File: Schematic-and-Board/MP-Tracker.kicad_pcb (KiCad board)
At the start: 2 copper layers, 61 parts, among them P1 DIL10, Q1 BC817, Q2 IRFR5303, Q3 BC817-40, Q4 IRFR5303, U1 MC34063, U2 TL082, U3 ATMEGA8-AI, U4 MC78L033, X1 3.6864MHz

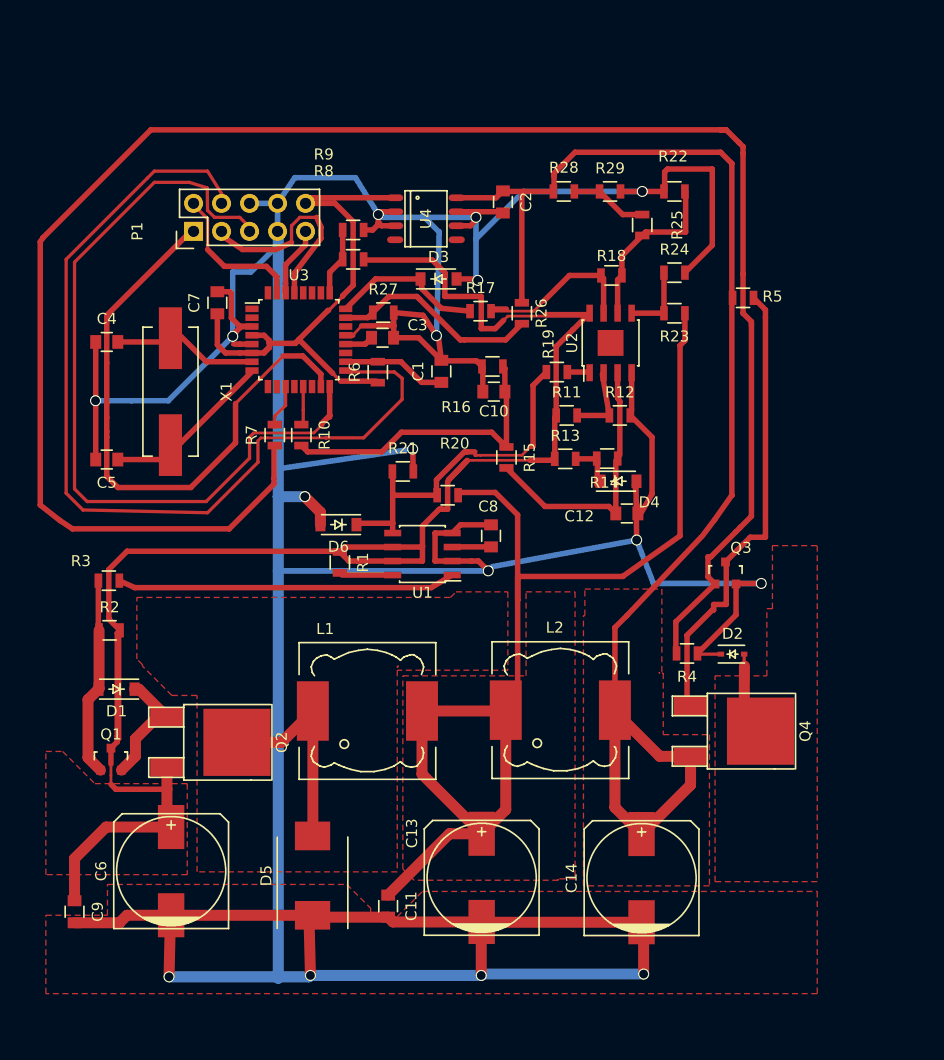
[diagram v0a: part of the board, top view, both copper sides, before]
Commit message: Update schematic and board design and firmware source.
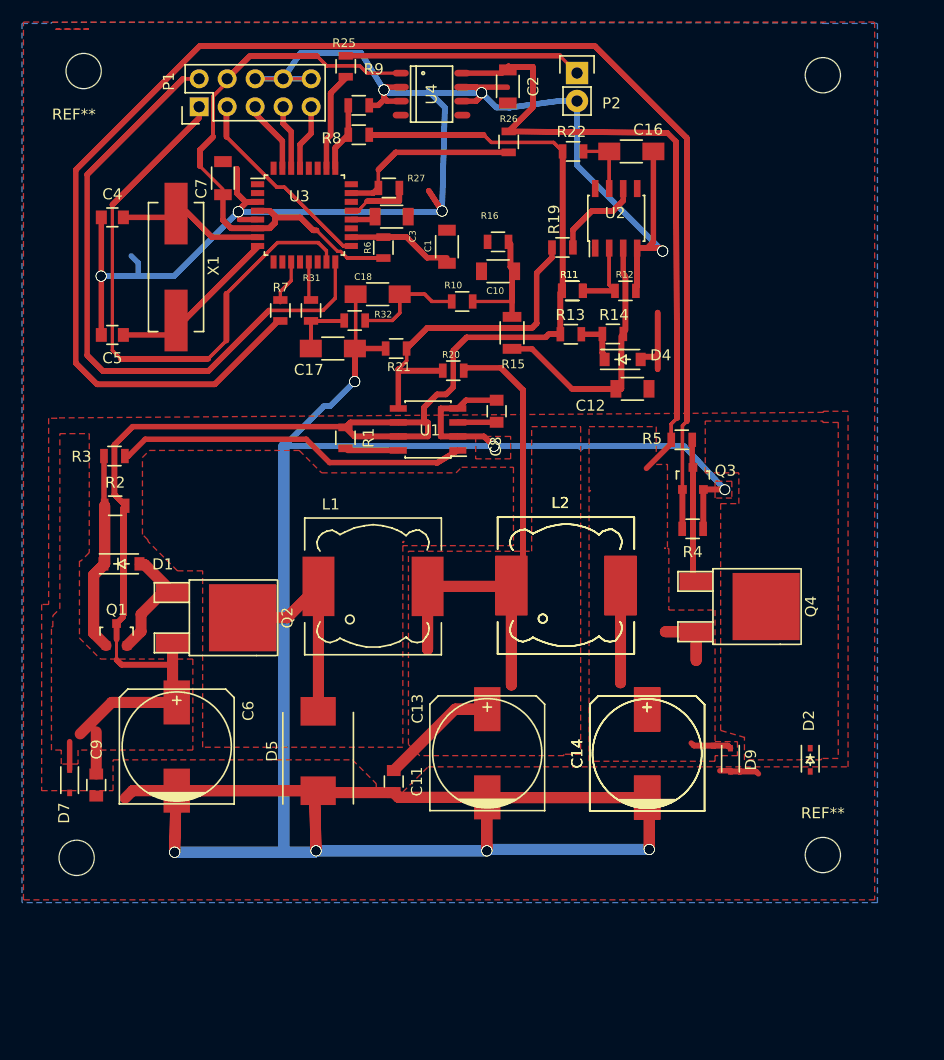
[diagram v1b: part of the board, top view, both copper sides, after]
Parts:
- removed D3, D6: 3V3, Diodes_SMD:SOD-123
- removed R17: 1k, Resistors_SMD:R_0805
- removed R18, R23, R24, R28, R29: 22k, Resistors_SMD:R_0805
- added ?: , Mounting_Holes:MountingHole_3.2mm_M3_DIN965, F.Cu at (167.6, 70.5)
- added ?: , Mounting_Holes:MountingHole_3.2mm_M3_DIN965, F.Cu at (99.9, 141.5)
- added C14: 330u, Capacitors_SMD:c_elec_10x10, F.Cu at (151.7, 132.0)
- added C16: 470n, Capacitors_SMD:C_1206_HandSoldering, F.Cu at (150.3, 77.4)
- added C17: 470n, Capacitors_SMD:C_1206_HandSoldering, F.Cu at (123.2, 95.3)
- added C18: 470n, Capacitors_SMD:C_1206_HandSoldering, F.Cu at (127.3, 90.3)
- added D7: 1N4001, Diodes_SMD:SOD-323, F.Cu at (99.3, 134.5)
- added D9: 1N4001, Diodes_SMD:SOD-323, F.Cu at (159.3, 132.6)
- added L2: 10u, Choke_SMD:Choke_SMD_12x12mm_h8mm, F.Cu at (144.3, 116.8)
- added P2: CON_2x1, Pin_Headers:Pin_Header_Straight_1x02, F.Cu at (145.3, 70.3)
- added R11: 22k, Resistors_SMD:R_0805, F.Cu at (144.9, 90.0)
- added R31: 1K, Resistors_SMD:R_0805, F.Cu at (121.2, 91.8)
- added R32: 1K, Resistors_SMD:R_0805, F.Cu at (125.2, 92.7)
- added REF**: , Mounting_Holes:MountingHole_3.2mm_M3_DIN965, F.Cu at (100.6, 70.1)
- added REF**: , Mounting_Holes:MountingHole_3.2mm_M3_DIN965, F.Cu at (167.6, 141.2)
- C1, C10, C2, C3, C7: value 100n -> 470n; footprint Capacitors_SMD:C_0805 -> Capacitors_SMD:C_1206
- C12: value 10n -> 470n; footprint Capacitors_SMD:C_0805 -> Capacitors_SMD:C_1206
- C8: value 1n5 -> 68p
- L1: value 22u -> 100u
- P1: value DIL10 -> (none)
- Q1: value BC817 -> BC817-40
- R1: value 180R -> 1k
- R12: value 3k9 -> 3k3
- R13: value 3K9 -> 10k
- R15: footprint Resistors_SMD:R_0805 -> Resistors_SMD:R_1206
- R19: value 3k9 -> 10k
- R20: value 47k -> 27k
- R21: value 4k4 -> 2k35
- R22: value 1M -> 47
- R25: value 2k2 -> 1K
- U2: value TL082 -> TL081
- U3: value ATMEGA8-AI -> ATMEGA8
- moved R25 30.5 mm to (124.4, 69.7)
- moved R10 19.0 mm to (134.9, 91.0), turned to 0 degrees
- moved R26 15.6 mm to (139.1, 76.5)
- moved R5 14.0 mm to (154.8, 103.6)
- moved D2 11.9 mm to (166.5, 132.6), turned to 270 degrees
- moved C9 11.7 mm to (101.7, 134.9)
- moved D1 11.4 mm to (104.0, 114.8), turned to 0 degrees
- moved C6 11.3 mm to (109.0, 131.4)
- moved R15 11.3 mm to (139.4, 93.9)
- moved R19 11.3 mm to (144.0, 86.1)
- moved R2 11.3 mm to (103.4, 109.5)
- moved R4 11.3 mm to (155.8, 111.6)
- moved R8 11.3 mm to (125.5, 75.9)
- moved C5 11.3 mm to (103.2, 94.0)
- moved C1 11.3 mm to (133.5, 86.0)
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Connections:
- D1 pad 1: Net-(D1-Pad1) -> Net-(D1-Pad2)
- D1 pad 2: Net-(D1-Pad2) -> Net-(D1-Pad1)
- D2 pad 1: GNDPWR -> VAA
- D2 pad 2: VAA -> GNDPWR
- P1 pad 10: +3.3V -> GNDPWR
- P1 pad 4: Net-(P1-Pad4) -> +3.3V
- P1 pad 7: GNDPWR -> Net-(P1-Pad7)
- R10 pad 1: Net-(R10-Pad1) -> Net-(C18-Pad1)
- R22 pad 1: Net-(R18-Pad2) -> VCC
- R22 pad 2: GNDPWR -> Net-(C16-Pad1)
- R25 pad 1: Net-(R18-Pad2) -> Net-(R25-Pad1)
- U2 pad 1: Net-(R19-Pad1) -> (no net)
- U2 pad 5: Net-(R23-Pad2) -> (no net)
- U2 pad 6: Net-(R18-Pad2) -> Net-(R19-Pad1)
- U2 pad 7: Net-(R17-Pad2) -> Net-(C16-Pad1)
- U2 pad 8: VCC -> (no net)
- U3 pad 1: Net-(U3-Pad1) -> (no net)
- U3 pad 10: Net-(U3-Pad10) -> (no net)
- U3 pad 12: Net-(U3-Pad12) -> (no net)
- U3 pad 13: Net-(R10-Pad1) -> Net-(R31-Pad1)
- U3 pad 14: Net-(U3-Pad14) -> (no net)
- U3 pad 16: Net-(P1-Pad5) -> Net-(P1-Pad2)
- U3 pad 17: Net-(P1-Pad4) -> Net-(P1-Pad3)
- U3 pad 19: Net-(U3-Pad19) -> (no net)
- U3 pad 2: Net-(U3-Pad2) -> (no net)
- U3 pad 22: Net-(U3-Pad22) -> (no net)
- U3 pad 24: Net-(D3-Pad1) -> (no net)
- U3 pad 26: Net-(U3-Pad26) -> Net-(R25-Pad1)
- U3 pad 27: Net-(U3-Pad27) -> (no net)
- U3 pad 28: Net-(U3-Pad28) -> (no net)
- U3 pad 29: Net-(P1-Pad3) -> Net-(P1-Pad9)
- U3 pad 30: Net-(P1-Pad9) -> Net-(P1-Pad7)
- U3 pad 31: Net-(P1-Pad2) -> Net-(P1-Pad5)
- U3 pad 32: Net-(U3-Pad32) -> (no net)
- U3 pad 9: Net-(U3-Pad9) -> (no net)
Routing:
- net GNDPWR: track 471.2 -> 756.0 mm, vias 16 -> 25
- net VCC: track 180.8 -> 282.0 mm
- net Net-(Q3-Pad1): track 169.8 -> 259.6 mm
- net Net-(P1-Pad2): track 13.5 -> 99.0 mm
- net Net-(P1-Pad4): track 84.9 -> 0.00 mm
- net Net-(P1-Pad5): track 74.4 -> 11.1 mm
- net Net-(P1-Pad1): track 54.3 -> 92.9 mm
- net +3.3V: track 59.7 -> 93.0 mm
- net +BATT: track 121.4 -> 147.9 mm
- net Net-(R19-Pad2): track 32.3 -> 51.6 mm
- net Net-(R17-Pad2): track 18.5 -> 0.00 mm
- net Net-(Q3-Pad3): track 42.3 -> 23.9 mm
- net Net-(P1-Pad3): track 19.6 -> 36.4 mm
- net Net-(C18-Pad1): track 0.00 -> 16.0 mm
- net Net-(R18-Pad2): track 15.7 -> 0.00 mm
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- added copper zone on B.Cu, net GNDPWR
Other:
- net class Small added: clearance 0.2, trace_width 0.2, via_dia 1, via_drill 0.8
- board text added: "3V3"
- board text added: "GND"
- board text added: "MISO"
- board text added: "MOSI"
- board text added: "RST"
- board text added: "RX"
- board text added: "SCL"
- board text added: "TX"
